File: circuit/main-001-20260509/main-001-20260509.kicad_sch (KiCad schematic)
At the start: 20 parts, among them J1 Conn_Relay, J2 Conn_Sub, Q1 BSS138, Q2 BSS138, SW1 RESET, U1 DEV-16771, U2 BNO055

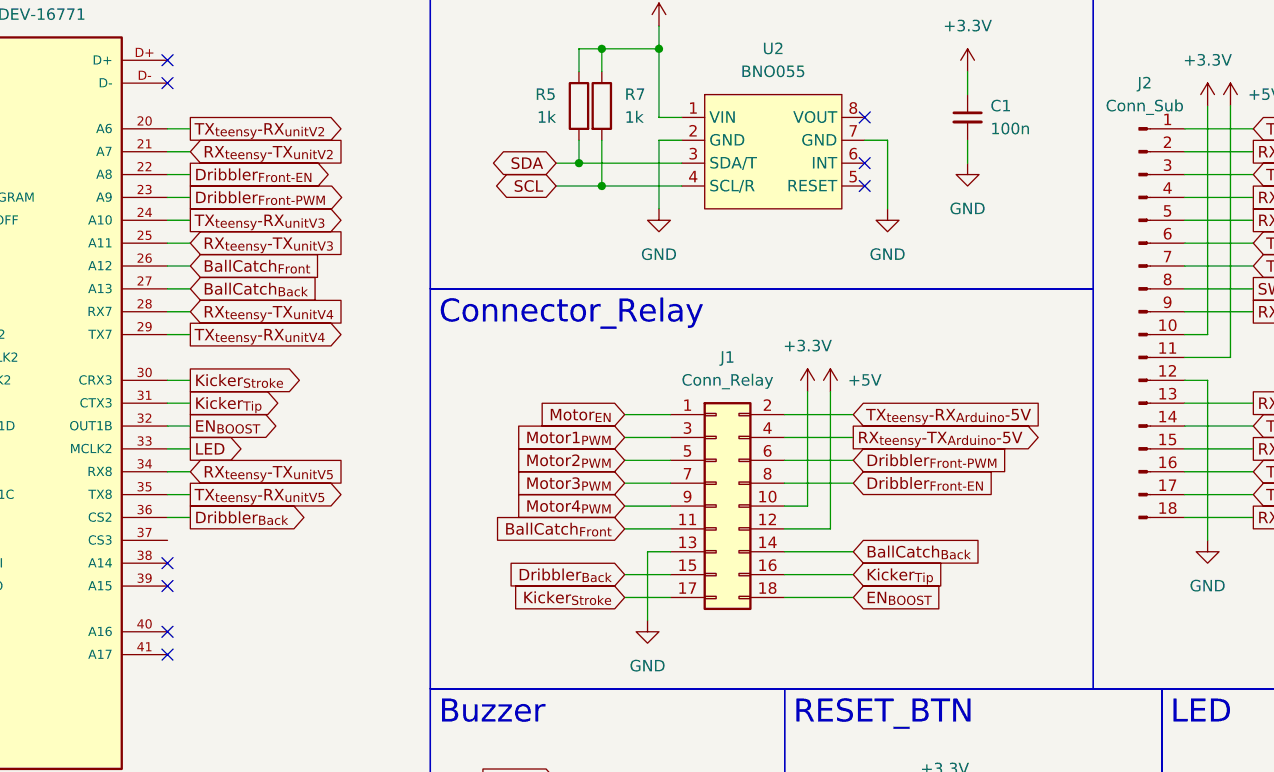
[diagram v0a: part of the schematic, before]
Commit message: Create 供給基板の回路図完成
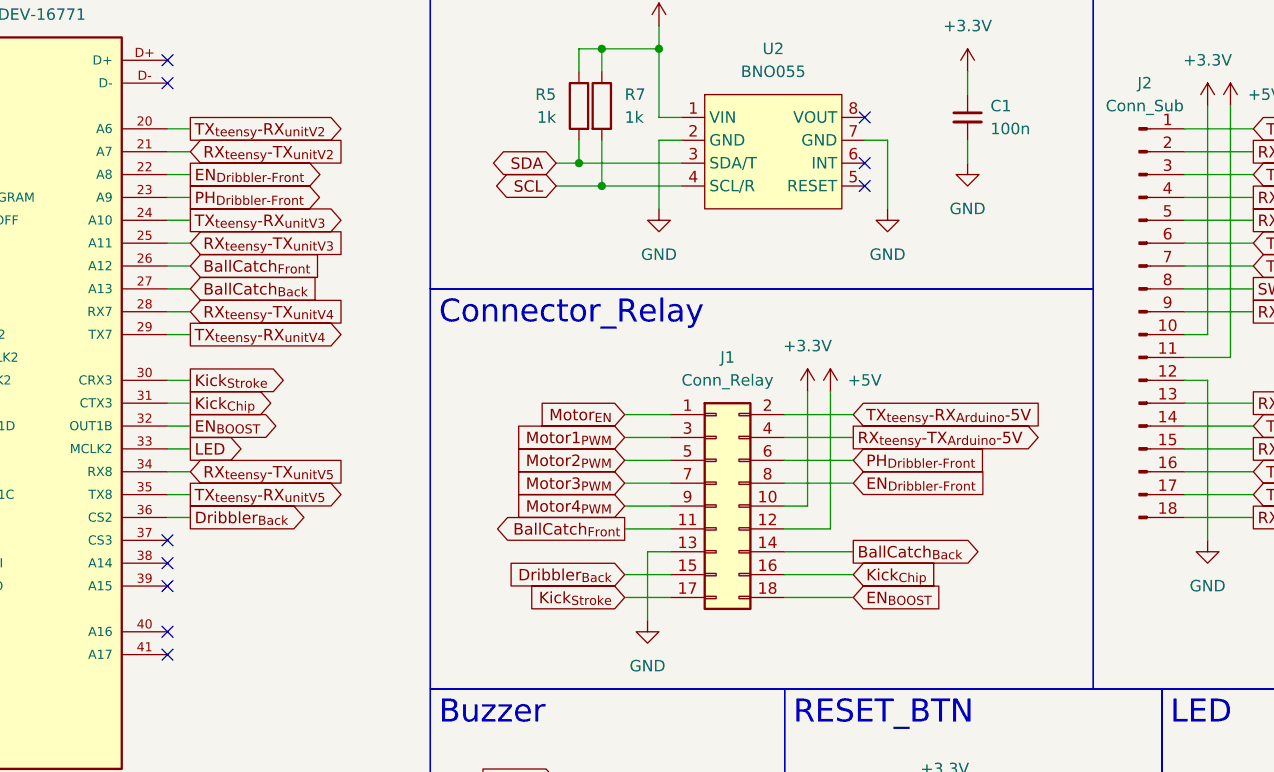
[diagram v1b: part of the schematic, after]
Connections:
- net Dribbler_{Front-EN} renamed EN_{Dribbler-Front}
- net Dribbler_{Front-PWM} renamed PH_{Dribbler-Front}
- net Kicker_{Stroke} renamed Kick_{Stroke}
- net Kicker_{Tip} renamed Kick_{Chip}
- no-connect marks 14 -> 15
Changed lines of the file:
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@@
+	)
+	(no_connect
+		(at 68.58 80.01)
 	)
 	(no_connect
@@
 		)
 	)
-	(global_label "Kicker_{Tip}"
+	(global_label "Kick_{Chip}"
 		(shape output)
 		(at 71.12 64.77 0)
@@
 		)
 		(property "Intersheetrefs" "${INTERSHEET_REFS}"
-			(at 82.166 64.77 0)
+			(at 79.5778 64.77 0)
 			(hide yes)
 			(show_name no)
@@
 	)
 	(global_label "BallCatch_{Back}"
-		(shape input)
+		(shape output)
 		(at 144.78 81.28 0)
 		(fields_autoplaced yes)
@@
 		)
 		(property "Intersheetrefs" "${INTERSHEET_REFS}"
-			(at 160.5763 81.28 0)
+			(at 157.6722 81.28 0)
 			(hide yes)
 			(show_name no)
@@
 		)
 	)
-	(global_label "Dribbler_{Front-PWM}"
-		(shape output)
-		(at 71.12 41.91 0)
-		(fields_autoplaced yes)
-		(effects
-			(font
-				(size 1.27 1.27)
-			)
-			(justify left)
-		)
-		(property "Intersheetrefs" "${INTERSHEET_REFS}"
-			(at 88.273 41.91 0)
-			(hide yes)
-			(show_name no)
-			(do_not_autoplace no)
-			(effects
-				(font
-					(size 1.27 1.27)
-				)
-				(justify left)
-			)
-		)
-	)
 	(global_label "Main_RST"
 		(shape output)
@@
 		)
 	)
-	(global_label "Kicker_{Stroke}"
+	(global_label "Kick_{Stroke}"
 		(shape output)
 		(at 71.12 62.23 0)
@@
 		)
 		(property "Intersheetrefs" "${INTERSHEET_REFS}"
-			(at 84.2926 62.23 0)
+			(at 80.5245 62.23 0)
 			(hide yes)
 			(show_name no)
@@
 		)
 	)
-	(global_label "Dribbler_{Front-PWM}"
+	(global_label "PH_{Dribbler-Front}"
 		(shape input)
 		(at 144.78 71.12 0)
@@
 		)
 		(property "Intersheetrefs" "${INTERSHEET_REFS}"
-			(at 163.83 71.12 0)
+			(at 157.0233 71.12 0)
 			(hide yes)
 			(show_name no)
@@
 		)
 	)
-	(global_label "Dribbler_{Front-EN}"
+	(global_label "EN_{Dribbler-Front}"
 		(shape output)
 		(at 71.12 39.37 0)
@@
 		)
 		(property "Intersheetrefs" "${INTERSHEET_REFS}"
-			(at 87.0086 39.37 0)
+			(at 83.3633 39.37 0)
 			(hide yes)
 			(show_name no)
@@
 		)
 	)
-	(global_label "Kicker_{Stroke}"
+	(global_label "Kick_{Stroke}"
 		(shape input)
 		(at 119.38 86.36 180)
@@
 		)
 		(property "Intersheetrefs" "${INTERSHEET_REFS}"
-			(at 105.6879 86.36 0)
+			(at 109.9755 86.36 0)
 			(hide yes)
 			(show_name no)
@@
 		)
 	)
-	(global_label "Dribbler_{Front-EN}"
+	(global_label "EN_{Dribbler-Front}"
 		(shape input)
 		(at 144.78 73.66 0)
@@
 		)
 		(property "Intersheetrefs" "${INTERSHEET_REFS}"
-			(at 162.4754 73.66 0)
+			(at 157.0233 73.66 0)
 			(hide yes)
 			(show_name no)
@@
 		)
 	)
+	(global_label "PH_{Dribbler-Front}"
+		(shape output)
+		(at 71.12 41.91 0)
+		(fields_autoplaced yes)
+		(effects
+			(font
+				(size 1.27 1.27)
+			)
+			(justify left)
+		)
+		(property "Intersheetrefs" "${INTERSHEET_REFS}"
+			(at 83.3633 41.91 0)
+			(hide yes)
+			(show_name no)
+			(do_not_autoplace no)
+			(effects
+				(font
+					(size 1.27 1.27)
+				)
+				(justify left)
+			)
+		)
+	)
 	(global_label "TX_{teensy}-RX_{Arduino}-3V3"
 		(shape input)
@@
 	)
 	(global_label "BallCatch_{Front}"
-		(shape input)
+		(shape output)
 		(at 119.38 78.74 180)
 		(fields_autoplaced yes)
@@
 		)
 		(property "Intersheetrefs" "${INTERSHEET_REFS}"
-			(at 103.2934 78.74 0)
+			(at 106.3613 78.74 0)
 			(hide yes)
 			(show_name no)
@@
 		)
 	)
-	(global_label "Kicker_{Tip}"
+	(global_label "Kick_{Chip}"
 		(shape input)
 		(at 144.78 83.82 0)
@@
 		)
 		(property "Intersheetrefs" "${INTERSHEET_REFS}"
-			(at 155.8594 83.82 0)
-			(hide yes)
-			(show_name no)
+			(at 153.2378 83.82 0)
+			(hide yes)
+			(show_name no)
